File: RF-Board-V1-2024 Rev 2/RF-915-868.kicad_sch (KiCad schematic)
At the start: 20 parts, among them J2 RFPC-SMA29-F, J3 RFPC-SMA29-F, SW3 SW_SPST, SW6 SW_SPST

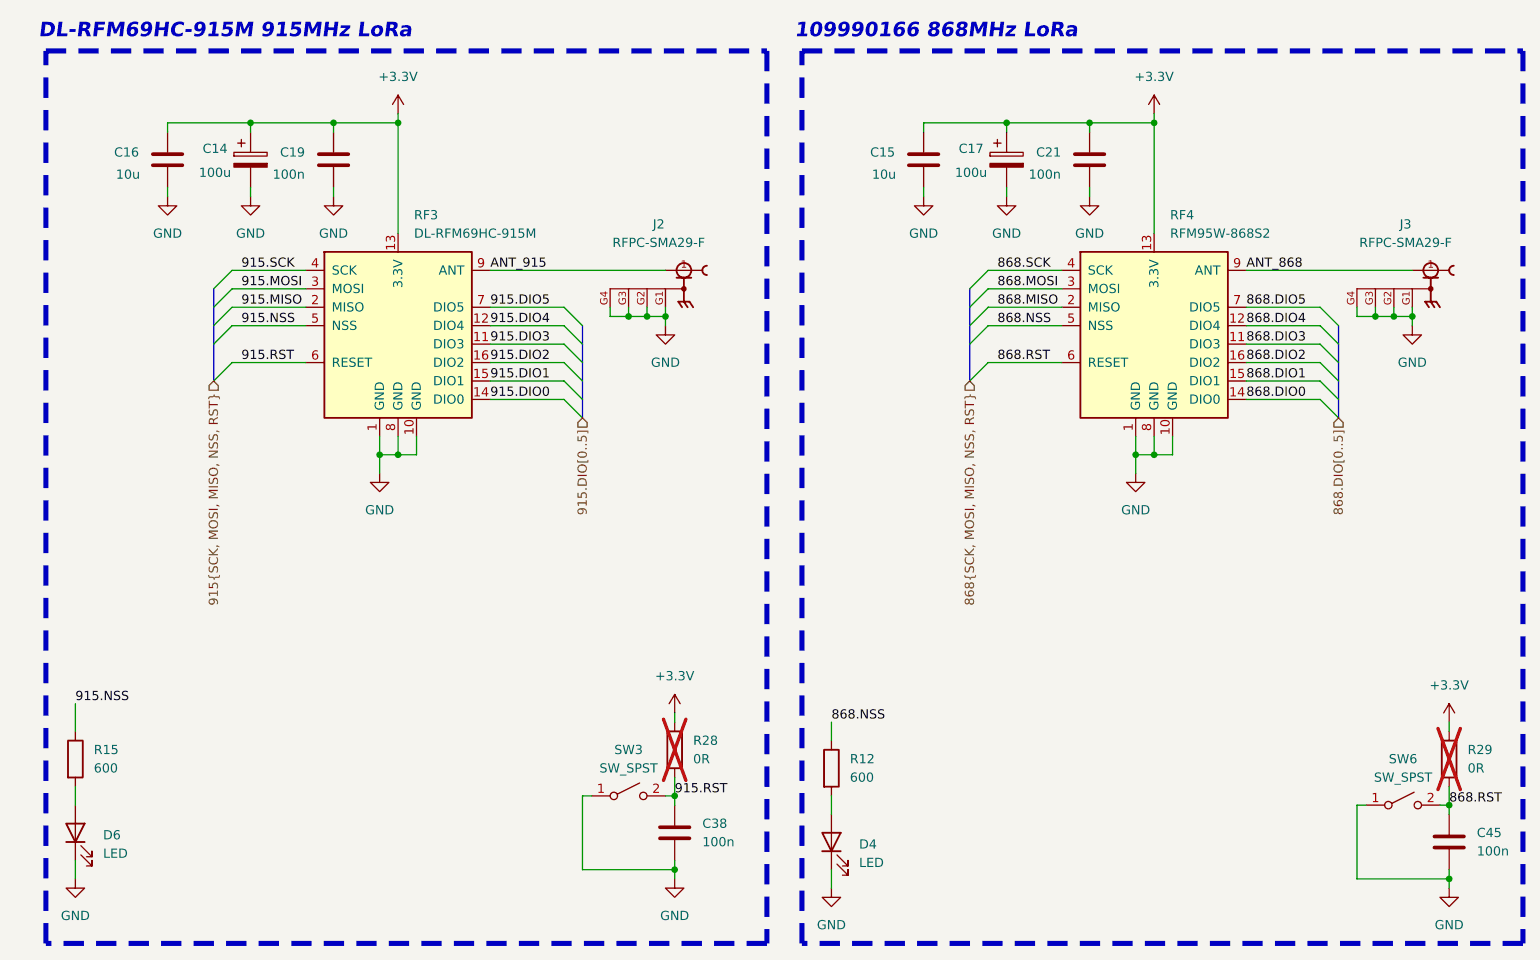
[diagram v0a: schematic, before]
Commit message: made some notes
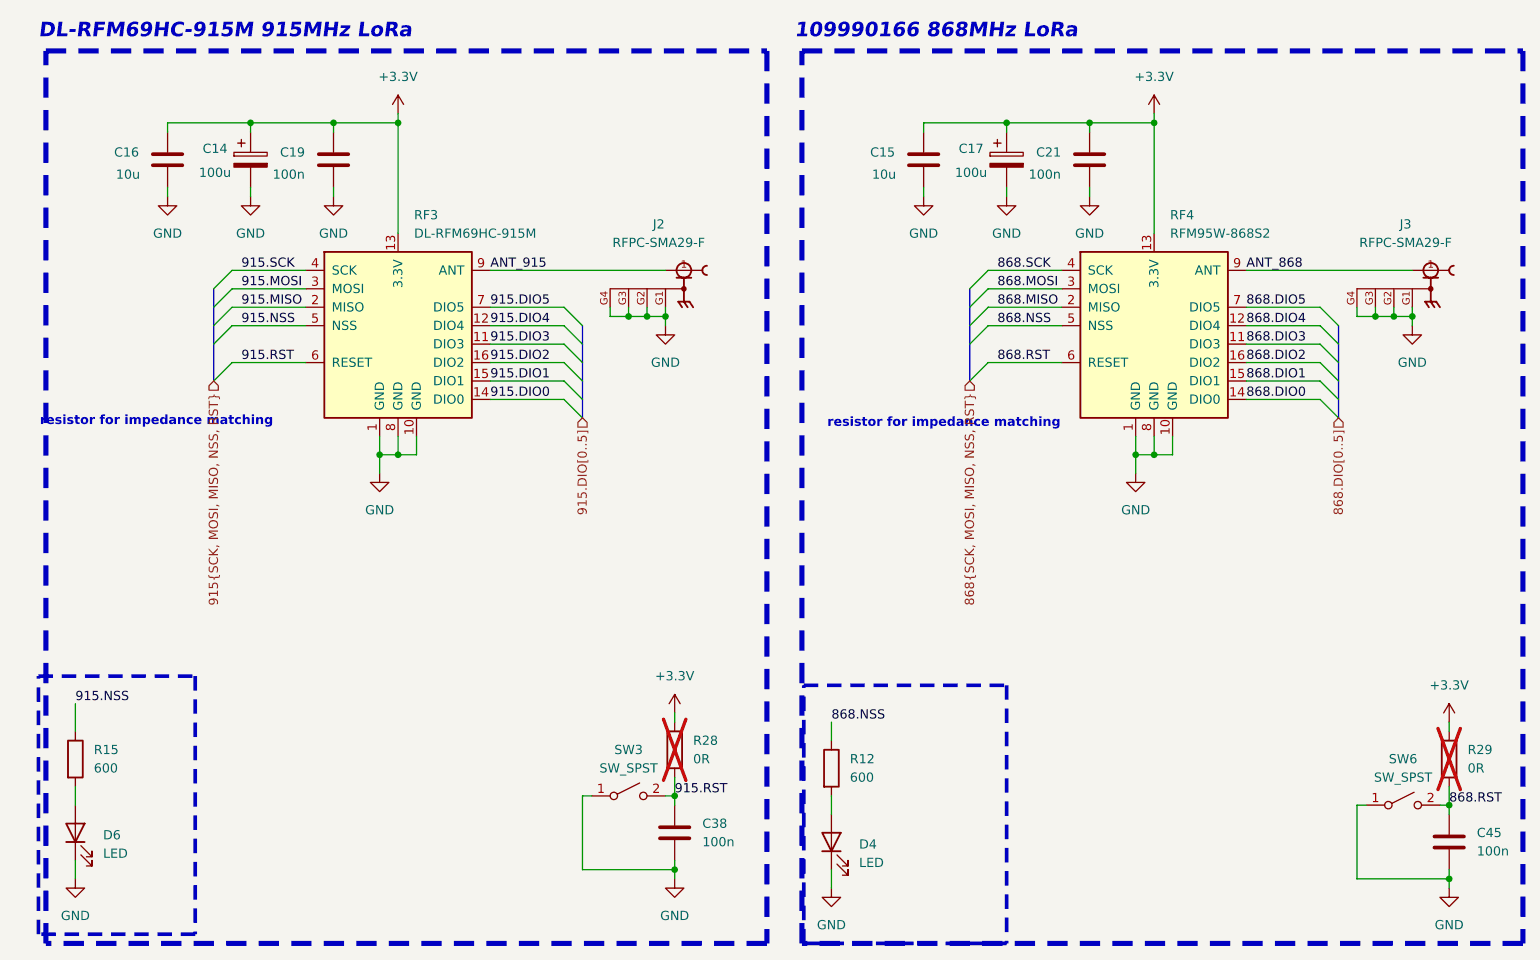
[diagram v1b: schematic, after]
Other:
- note added: "resistor for impedance matching"
